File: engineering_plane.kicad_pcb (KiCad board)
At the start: 2 copper layers, 100 x 70 mm, 100 parts, among them IC1 LP5907MFX-3.3_NOPB, IC2 BMI270, IC3 MMC5983MA, J1 Conn_01x02_Pin, J10 JST_1mm_4, J11 171857-0003, J12 171857-0003, J13 171857-0003, J14 171857-0003, J15 502570-0893, J2 Conn_01x04_Pin, J3 Conn_01x04_Pin, J4 Conn_01x03, J5 JST_1mm_4, J6 Conn_01x01_Pin, J7 Conn_01x01_Pin, J8 JST_1mm_4, J9 JST_1mm_4, U1 BMP581, U2 TPS54302DDCR, U3 TPS54302DDCR

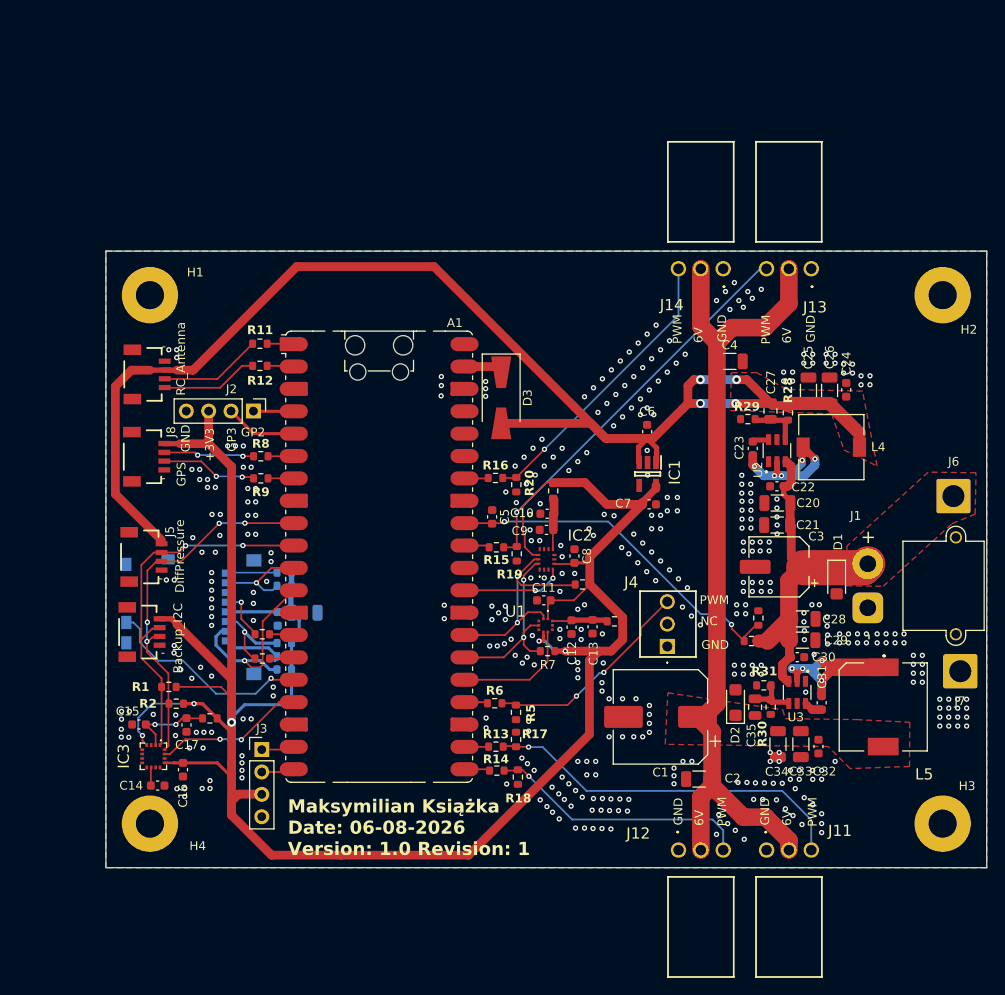
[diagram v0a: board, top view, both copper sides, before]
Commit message: Revised componenents, need to route
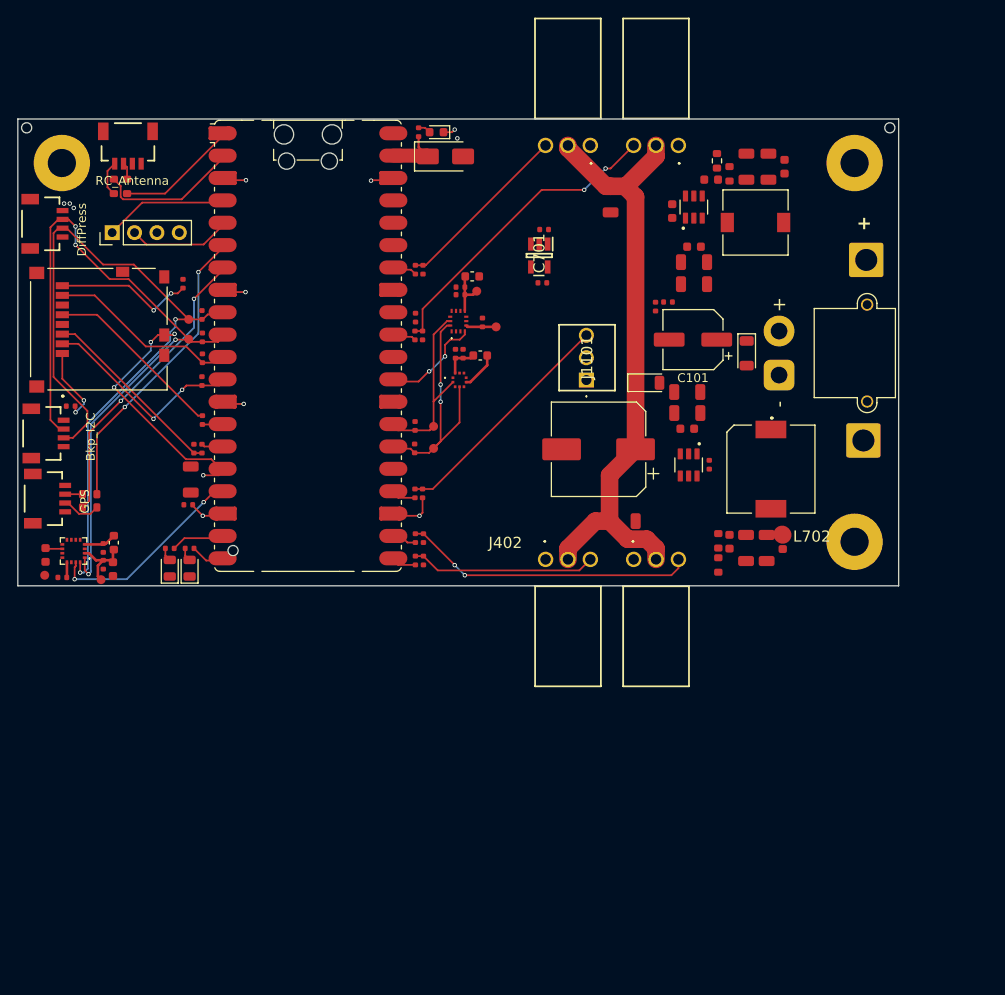
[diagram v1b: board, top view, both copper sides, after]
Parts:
- removed A1: RaspberryPi_Pico_W, Module:RaspberryPi_Pico_Common_SMD
- removed C1: 470u, Capacitor_SMD:CP_Elec_10x10.5
- removed C10, C13, C16, C6, C7: 1u, Capacitor_SMD:C_0603_1608Metric
- removed C11, C12, C15, C19, C5, C8, C9: 100n, Capacitor_SMD:C_0603_1608Metric
- removed C14, C17: 10u, Capacitor_SMD:C_0603_1608Metric
- removed C18, C25, C26, C33, C34: 22u, Capacitor_SMD:C_1206_3216Metric
- removed C2, C20, C21, C28, C29, C4: 10u, Capacitor_SMD:C_1206_3216Metric
- removed C22, C23, C24, C30, C31, C32: 0.1u, Capacitor_SMD:C_0603_1608Metric
- removed C27, C35: 100p, Capacitor_SMD:C_0805_2012Metric
- removed C3: 100u, Capacitor_SMD:CP_Elec_6.3x7.7
- removed D1: SMF15A, Diode_SMD:D_SMF
- removed D2: SMF6V5A, Diode_SMD:D_SMF
- removed D3: SS24, Diode_SMD:D_SMA-SMB_Universal_Handsoldering
- removed H4: MountingHole_Pad, MountingHole:MountingHole_3.2mm_M3_Pad
- removed IC1: LP5907MFX-3.3_NOPB, eng_plane_lib:SOT95P280X145-5M
- removed IC2: BMI270, eng_plane_lib:BMI270
- removed J10, J5, J8, J9: JST_1mm_4, PCM_SparkFun-Connector:JST_1x04_P1.0mm_Horizontal_SMD
- removed J2, J3: Conn_01x04_Pin, Connector_PinHeader_2.54mm:PinHeader_1x04_P2.54mm_Vertical
- removed J4: Conn_01x03, eng_plane_lib:1718564003
- removed J6, J7: Conn_01x01_Pin, Connector_Wire:SolderWire-2sqmm_1x01_D2mm_OD3.9mm
- removed L1, L2, L3: 600 Ohm, PCM_SparkFun-Resistor:R_0603_1608Metric
- removed L4: 10u, Inductor_SMD:L_7.3x7.3_H4.5
- removed R1, R10, R2, R7: 4.7k, PCM_SparkFun-Resistor:R_0603_1608Metric
- removed R11, R12, R13, R14, R15, R16, R21, R23, R6, R8, R9: 22, PCM_SparkFun-Resistor:R_0603_1608Metric
- removed R17, R18, R19, R20, R22, R24, R25, R26, R27, R4, R5: 10k, PCM_SparkFun-Resistor:R_0603_1608Metric
- removed R28, R30: 100k, PCM_SparkFun-Resistor:R_0603_1608Metric
- removed R29: 13.3k, PCM_SparkFun-Resistor:R_0603_1608Metric
- removed R3: 47k, PCM_SparkFun-Resistor:R_0603_1608Metric
- removed R31: 11k, PCM_SparkFun-Resistor:R_0603_1608Metric
- removed U2, U3: TPS54302DDCR, eng_plane_lib:SOT95P280X110-6N
- added A801: RaspberryPi_Pico_W, Module:RaspberryPi_Pico_Common_SMD, F.Cu at (132.9, 75.8)
- added C101: 100u, Capacitor_SMD:CP_Elec_6.3x7.7, F.Cu at (176.7, 75.0)
- added C102: 100nF, PCM_JLCPCB:C_0402, F.Cu at (145.2, 72.5)
- added C103: 470u, Capacitor_SMD:CP_Elec_10x10.5, F.Cu at (165.9, 87.5)
- added C104: 10uF, PCM_JLCPCB:C_1206, F.Cu at (168.7, 95.7)
- added C105: 10uF, PCM_JLCPCB:C_1206, F.Cu at (167.3, 59.1)
- added C201: 100nF, PCM_JLCPCB:C_0402, F.Cu at (152.8, 73.1)
- added C202: 100nF, PCM_JLCPCB:C_0402, F.Cu at (150.2, 69.1)
- added C203: 1uF, PCM_JLCPCB:C_0402, F.Cu at (150.2, 69.9)
- added C301: 100nF, PCM_JLCPCB:C_0402, F.Cu at (105.0, 102.0)
- added C302: 100nF, PCM_JLCPCB:C_0402, F.Cu at (149.7, 76.7)
- added C303: 1uF, PCM_JLCPCB:C_0402, F.Cu at (150.6, 76.7)
- added C501: 10uF, PCM_JLCPCB:C_0603, F.Cu at (103.1, 99.5)
- added C502: 100nF, PCM_JLCPCB:C_0402, F.Cu at (109.7, 100.6)
- added C503: 1uF, PCM_JLCPCB:C_0402, F.Cu at (109.7, 98.7)
- added C504: 10uF, PCM_JLCPCB:C_0603, F.Cu at (110.8, 101.1)
- added C601: 22uF, PCM_JLCPCB:C_1206, F.Cu at (119.6, 90.9)
- added C602: 100nF, PCM_JLCPCB:C_0402, F.Cu at (119.3, 93.8)
- added C701: 10uF, PCM_JLCPCB:C_1206, F.Cu at (176.8, 68.8)
- added C702: 10uF, PCM_JLCPCB:C_1206, F.Cu at (176.8, 66.2)
- added C703: 100nF, PCM_JLCPCB:C_0603, F.Cu at (176.8, 64.5)
- added C704: 1uF, PCM_JLCPCB:C_0402, F.Cu at (159.8, 62.5)
- added C705: 100nF, PCM_JLCPCB:C_0603, F.Cu at (174.3, 60.5)
- added C706: 1uF, PCM_JLCPCB:C_0402, F.Cu at (159.6, 68.6)
- added C707: 100nF, PCM_JLCPCB:C_0603, F.Cu at (187.0, 55.4)
- added C708: 22uF, PCM_JLCPCB:C_1206, F.Cu at (185.2, 55.4)
- added C709: 22uF, PCM_JLCPCB:C_1206, F.Cu at (182.7, 55.4)
- added C710: 100pF, PCM_JLCPCB:C_0603, F.Cu at (178.7, 56.9)
- added C711: 10uF, PCM_JLCPCB:C_1206, F.Cu at (176.0, 81.0)
- added C712: 10uF, PCM_JLCPCB:C_1206, F.Cu at (176.0, 83.4)
- added C713: 100nF, PCM_JLCPCB:C_0603, F.Cu at (176.0, 85.2)
- added C714: 100nF, PCM_JLCPCB:C_0402, F.Cu at (178.5, 89.2)
- added C715: 100nF, PCM_JLCPCB:C_0603, F.Cu at (186.8, 98.0)
- added C716: 22uF, PCM_JLCPCB:C_1206, F.Cu at (182.7, 98.7)
- added C717: 22uF, PCM_JLCPCB:C_1206, F.Cu at (185.0, 98.7)
- added C718: 100pF, PCM_JLCPCB:C_0603, F.Cu at (180.8, 98.0)
- added D101: SMF15A, PCM_JLCPCB:D_SOD-123FL, F.Cu at (182.8, 76.6)
- added D102: SMF6.5A, PCM_JLCPCB:D_SOD-123FL, F.Cu at (171.4, 80.0)
- added D801: Red, PCM_JLCPCB:D_0805, F.Cu at (117.2, 101.0)
- added D802: Green, PCM_JLCPCB:D_0805, F.Cu at (119.5, 101.0)
- added D803: SS24, PCM_JLCPCB:D_SMA, F.Cu at (148.6, 54.2)
- added D804: Yellow, PCM_JLCPCB:D_0603, F.Cu at (147.5, 51.5)
- added FB201: ~, PCM_JLCPCB:FB_0603, F.Cu at (151.6, 67.9)
- added FB301: ~, PCM_JLCPCB:FB_0603, F.Cu at (152.5, 76.8)
- added FB501: ~, PCM_JLCPCB:FB_0603, F.Cu at (110.9, 98.1)
- added H102: ~, PCM_JLCPCB:Hole_Tooling_JLCPCB, F.Cu at (124.4, 99.0)
- added H103: ~, PCM_JLCPCB:Hole_Tooling_JLCPCB, F.Cu at (199.0, 51.0)
- added H104: ~, PCM_JLCPCB:Hole_Tooling_JLCPCB, F.Cu at (101.0, 51.0)
- added IC201: BMI270, eng_plane_lib:BMI270, F.Cu at (150.0, 73.0)
- added IC701: LP5907MFX-3.3_NOPB, eng_plane_lib:SOT95P280X145-5M, F.Cu at (159.2, 65.5)
- added J1001: JST_1mm_4, PCM_SparkFun-Connector:JST_1x04_P1.0mm_Horizontal_SMD, F.Cu at (112.5, 55.1)
- added J102: Conn_01x01_Pin, Connector_Wire:SolderWire-2sqmm_1x01_D2mm_OD3.9mm, F.Cu at (196.3, 66.0)
- added J103: Conn_01x01_Pin, Connector_Wire:SolderWire-2sqmm_1x01_D2mm_OD3.9mm, F.Cu at (196.0, 86.5)
- added J1101: Conn_01x03, eng_plane_lib:1718564003, F.Cu at (164.6, 79.6)
- added J1201: JST_1mm_4, PCM_SparkFun-Connector:JST_1x04_P1.0mm_Horizontal_SMD, F.Cu at (105.1, 61.9)
- added J1301: JST_1mm_4, PCM_SparkFun-Connector:JST_1x04_P1.0mm_Horizontal_SMD, F.Cu at (105.2, 85.7)
- added J801: Conn_01x04_Pin, Connector_PinHeader_2.54mm:PinHeader_1x04_P2.54mm_Vertical, F.Cu at (110.7, 62.9)
- added J901: JST_1mm_4, PCM_SparkFun-Connector:JST_1x04_P1.0mm_Horizontal_SMD, F.Cu at (105.4, 93.1)
- added L701: 10u, Inductor_SMD:L_7.3x7.3_H4.5, F.Cu at (183.8, 61.8)
- added R1001: 22Ω, PCM_JLCPCB:R_0603, F.Cu at (112.4, 57.6)
- added R1002: 22Ω, PCM_JLCPCB:R_0603, F.Cu at (110.9, 57.6)
- added R101: 47kΩ, PCM_JLCPCB:R_0402, F.Cu at (173.8, 70.8)
- added R102: 10kΩ, PCM_JLCPCB:R_0402, F.Cu at (172.4, 71.3)
- added R1101: 10kΩ, PCM_JLCPCB:R_0402, F.Cu at (145.9, 92.5)
- added R1102: 22Ω, PCM_JLCPCB:R_0402, F.Cu at (145.1, 92.5)
- added R401: 22Ω, PCM_JLCPCB:R_0402, F.Cu at (145.1, 97.6)
- added R402: 22Ω, PCM_JLCPCB:R_0402, F.Cu at (145.1, 100.1)
- added R403: 22Ω, PCM_JLCPCB:R_0402, F.Cu at (145.1, 74.6)
- added R404: 22Ω, PCM_JLCPCB:R_0402, F.Cu at (145.1, 67.1)
- added R405: 10kΩ, PCM_JLCPCB:R_0402, F.Cu at (146.1, 97.6)
- added R406: 10kΩ, PCM_JLCPCB:R_0402, F.Cu at (146.1, 100.1)
- added R407: 10kΩ, PCM_JLCPCB:R_0402, F.Cu at (145.9, 74.6)
- added R408: 10kΩ, PCM_JLCPCB:R_0402, F.Cu at (146.0, 67.1)
- added R601: 22Ω, PCM_JLCPCB:R_0402, F.Cu at (120.9, 87.4)
- added R602: 10kΩ, PCM_JLCPCB:R_0402, F.Cu at (120.0, 87.4)
- added R603: 22Ω, PCM_JLCPCB:R_0402, F.Cu at (121.0, 84.2)
- added R604: 10kΩ, PCM_JLCPCB:R_0402, F.Cu at (120.9, 79.8)
- added R605: 10kΩ, PCM_JLCPCB:R_0402, F.Cu at (121.0, 77.2)
- added R606: 10kΩ, PCM_JLCPCB:R_0402, F.Cu at (106.0, 82.6)
- added R607: 10kΩ, PCM_JLCPCB:R_0402, F.Cu at (118.8, 68.7)
- added R701: 100kΩ, PCM_JLCPCB:R_0603, F.Cu at (180.8, 56.2)
- added R702: 13.3k, PCM_SparkFun-Resistor:R_0603_1608Metric, F.Cu at (179.4, 54.8)
- added R703: 100kΩ, PCM_JLCPCB:R_0603, F.Cu at (179.5, 97.9)
- added R704: 11kΩ, PCM_JLCPCB:R_0603, F.Cu at (179.5, 100.6)
- added R801: 4.7kΩ, PCM_JLCPCB:R_0402, F.Cu at (121.0, 74.8)
- added R802: 4.7kΩ, PCM_JLCPCB:R_0402, F.Cu at (120.9, 72.2)
- added R803: 1kΩ, PCM_JLCPCB:R_0402, F.Cu at (117.2, 98.8)
- added R804: 1kΩ, PCM_JLCPCB:R_0402, F.Cu at (119.5, 98.8)
- added R805: 2.2kΩ, PCM_JLCPCB:R_0402, F.Cu at (145.5, 51.5)
- added R806: 4.7kΩ, PCM_JLCPCB:R_0402, F.Cu at (145.1, 87.4)
- added R807: 4.7kΩ, PCM_JLCPCB:R_0402, F.Cu at (145.1, 84.8)
- added R901: 22Ω, PCM_JLCPCB:R_0603, F.Cu at (108.2, 92.6)
- added R902: 22Ω, PCM_JLCPCB:R_0603, F.Cu at (108.2, 94.1)
- added TP201: 1.0mm, PCM_SparkFun-Connector:TestPoint-1.0mm, F.Cu at (154.3, 73.6)
- added TP202: 1.0mm, PCM_SparkFun-Connector:TestPoint-1.0mm, F.Cu at (152.1, 69.5)
- added TP501: 1.0mm, PCM_SparkFun-Connector:TestPoint-1.0mm, F.Cu at (103.0, 101.8)
- added TP502: 1.0mm, PCM_SparkFun-Connector:TestPoint-1.0mm, F.Cu at (109.5, 102.3)
- added TP801: 1.0mm, PCM_SparkFun-Connector:TestPoint-1.0mm, F.Cu at (119.4, 72.8)
- added TP802: 1.0mm, PCM_SparkFun-Connector:TestPoint-1.0mm, F.Cu at (119.4, 75.0)
- added TP803: 1.0mm, PCM_SparkFun-Connector:TestPoint-1.0mm, F.Cu at (147.2, 87.4)
- added TP804: 1.0mm, PCM_SparkFun-Connector:TestPoint-1.0mm, F.Cu at (147.2, 84.9)
- added U701: TPS54302DDCR, eng_plane_lib:SOT95P280X110-6N, F.Cu at (176.8, 60.0)
- added U702: TPS54302DDCR, eng_plane_lib:SOT95P280X110-6N, F.Cu at (176.2, 89.3)
- J601: renamed from J15; moved to F.Cu
- moved J401 36.3 mm to (169.9, 100.0)
- moved J402 36.3 mm to (159.9, 100.0)
- moved J601 34.3 mm to (109.2, 73.9)
- moved H106 33.5 mm to (195.0, 98.0)
- moved L702 29.9 mm to (185.5, 89.8)
- moved U301 29.5 mm to (150.2, 79.6), turned to 0 degrees
- moved J101 28.3 mm to (186.4, 79.1)
- moved IC501 25.0 mm to (106.3, 99.0), turned to -90 degrees
- moved J403 20.6 mm to (175.0, 53.0)
- moved J404 20.6 mm to (165.0, 53.0)
- moved H101 18.0 mm to (105.0, 55.0)
- moved H105 18.0 mm to (195.0, 55.0)
- renumbered H1 to H101, H2 to H105, H3 to H106, IC3 to IC501, J1 to J101, J11 to J401, J12 to J402, J13 to J403, J14 to J404, L5 to L702, U1 to U301
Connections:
- IC501 pad 1: /i2c1_scl -> /BackupMag/I2C.SCL
- IC501 pad 15: /mmc_int -> /MCU/mmc_int
- IC501 pad 16: /i2c1_sda -> /BackupMag/I2C.SDA
- J601 pad 2: /spi1_cs -> /MCU/sd_cs
- J601 pad 7: /spi1_rx -> /MCU/SPI1.MISO
- J601 pad DS1: /sd_int -> /MCU/sd_int
- U301 pad 2: /i2c0_scl -> /MCU/I2C0.SCL
- U301 pad 4: /i2c0_sda -> /MCU/I2C0.SDA
- U301 pad 7: /bmp_int -> /MCU/bmp_int
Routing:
- net +3V3: track 268.7 -> 13.2 mm, vias 5 -> 0
- net +5V: track 154.4 -> 0.00 mm
- net /BackupMag/I2C.SDA: track 0.00 -> 86.7 mm, vias 0 -> 2
- net /BackupMag/I2C.SCL: track 0.00 -> 85.3 mm, vias 0 -> 4
- net VBATT: track 45.0 -> 0.00 mm
- net /i2c1_scl: track 42.3 -> 0.00 mm, vias 2 -> 0
- net /i2c1_sda: track 42.0 -> 0.00 mm, vias 4 -> 0
- net /adc_v: track 40.3 -> 0.00 mm, vias 2 -> 0
- net /GPS/UART.RX: track 0.00 -> 35.2 mm, vias 0 -> 2
- net /GPS/UART.TX: track 0.00 -> 34.0 mm, vias 0 -> 2
- net /MCU/sd_int: track 0.00 -> 28.9 mm, vias 0 -> 4
- net /MCU/I2C0.SDA: track 0.00 -> 28.1 mm, vias 0 -> 2
- net Net-(J1101-Pin_3): track 0.00 -> 26.7 mm
- net +6V: track 95.0 -> 69.6 mm
- net /i2c0_scl: track 24.9 -> 0.00 mm, vias 2 -> 0
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- added copper zone on In2.Cu, net +3V3
- added copper zone on In2.Cu, net +5V
- added copper zone on In1.Cu, net GND
- added copper zone on In2.Cu, net VBATT
- removed copper zone on F.Cu, net +5V
- removed copper zone on F.Cu, net +6V
- removed copper zone on B.Cu, net GND
- removed copper zone on F.Cu, net GND
- removed copper zone on F.Cu, net VBATT
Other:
- board size 100 x 70 mm -> 100 x 53 mm
- copper layers 2 -> 4
- board text added: "+"
- board text added: "Bkp_I2C"
- board text added: "DiffPress"
- board text removed: "+3V3"
- board text removed: "-"
- board text removed: "6V"
- board text removed: "Backup_I2C"
- board text removed: "DiffPressure"
- board text removed: "GND"
- board text removed: "GP2"
- board text removed: "GP3"
- board text removed: "Maksymilian Książka Date: 06-08-2026 Version: 1.0 Revision: 1"
- board text removed: "NC"
- board text removed: "PWM"
